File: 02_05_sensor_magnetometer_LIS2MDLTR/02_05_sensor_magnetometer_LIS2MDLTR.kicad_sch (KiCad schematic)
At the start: 13 parts, among them J1 MICROMOD-2222, U2 AP2112K-3.3, U3 LIS2MDLTR

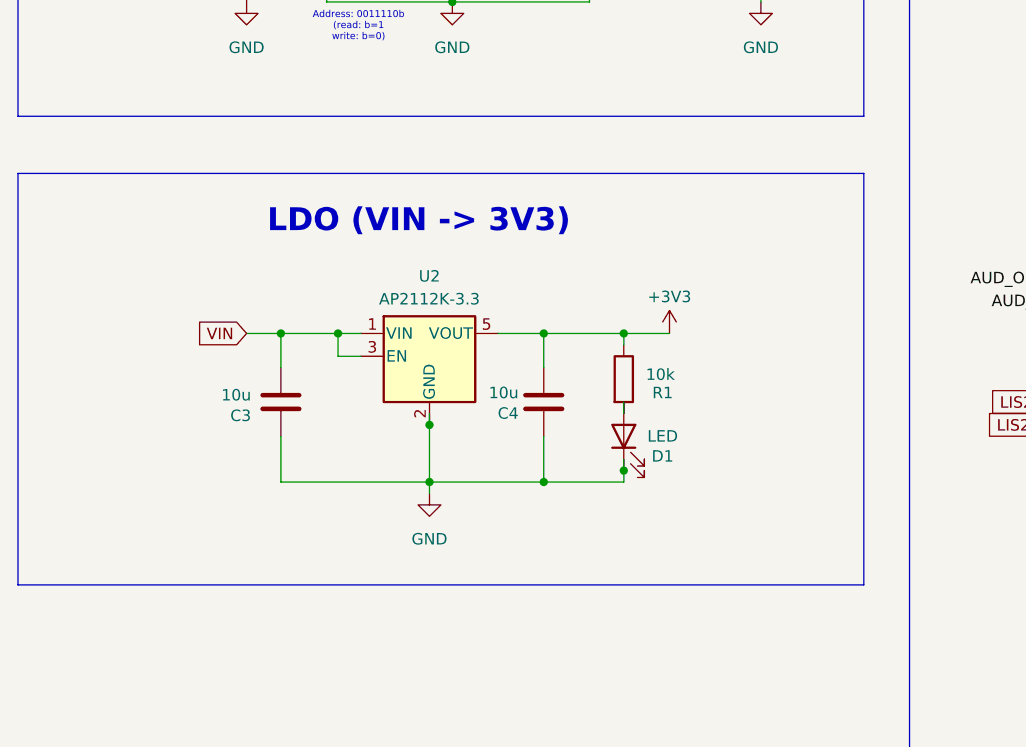
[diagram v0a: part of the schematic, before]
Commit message: filled missing connections :/
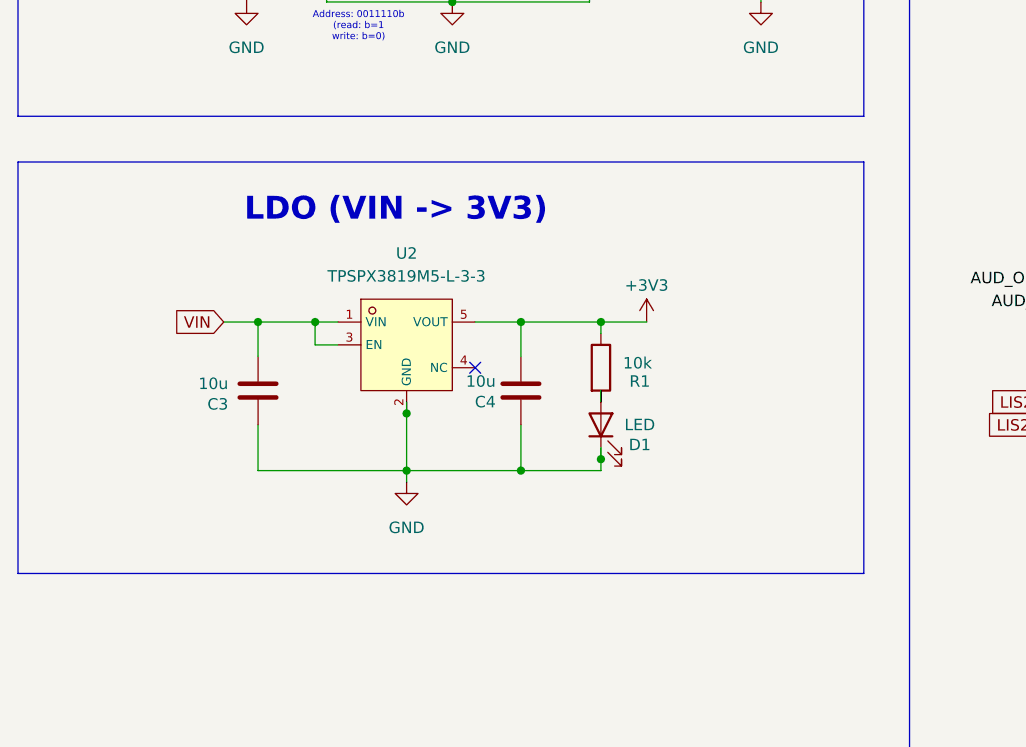
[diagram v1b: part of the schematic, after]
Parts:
- removed U2: AP2112K-3.3, Package_TO_SOT_SMD:SOT-23-5, symbol Regulator_Linear:AP2112K-3.3
- added U2: TPSPX3819M5-L-3-3, TPSPX3819M5-L-3-3:SOT-23-5_L3.0-W1.6-P0.95-LS2.8-BR, symbol TPSPX3819M5-L-3-3:TPSPX3819M5-L-3-3
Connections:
- net +3V3: now also U2.5 (VOUT)
- net GND: now also U2.2 (GND)
- net VIN: now also U2.1 (VIN), U2.3 (EN)
- no-connect marks 56 -> 57
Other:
- moved on the sheet: C3, C4, D1, R1
